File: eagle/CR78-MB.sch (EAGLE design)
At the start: 29 parts, among them IC1 40106N, Q1 2N3904, Q510 2N3904, Q518 2N3904, Q7 2N3904

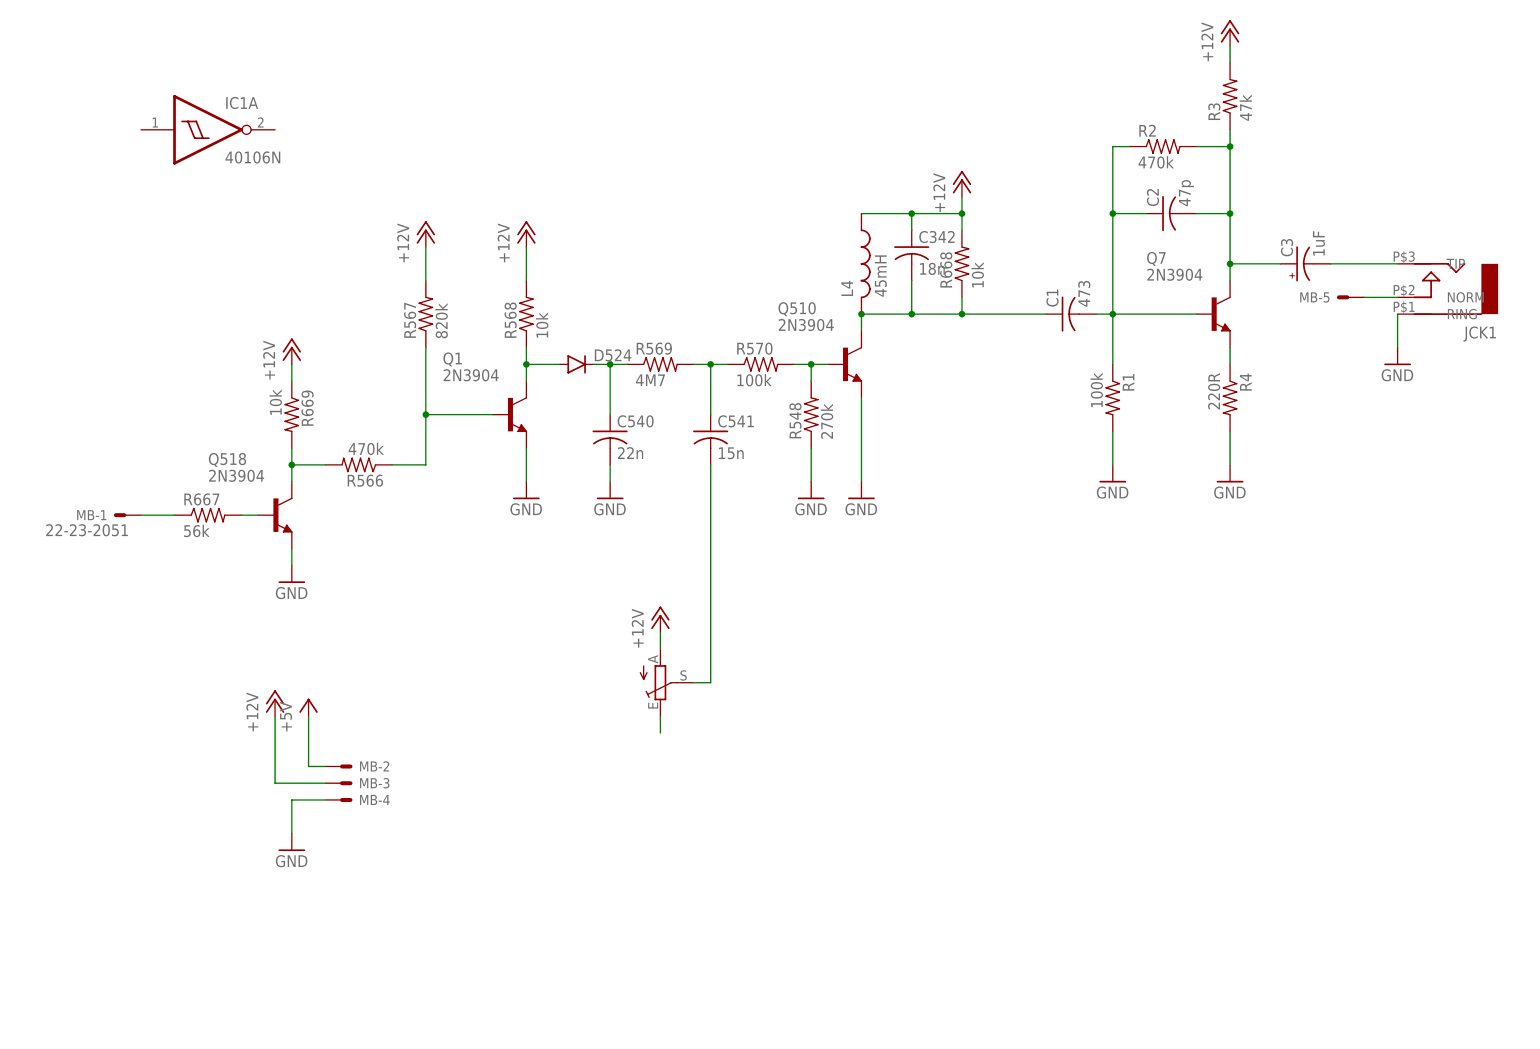
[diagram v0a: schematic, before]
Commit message: schemo
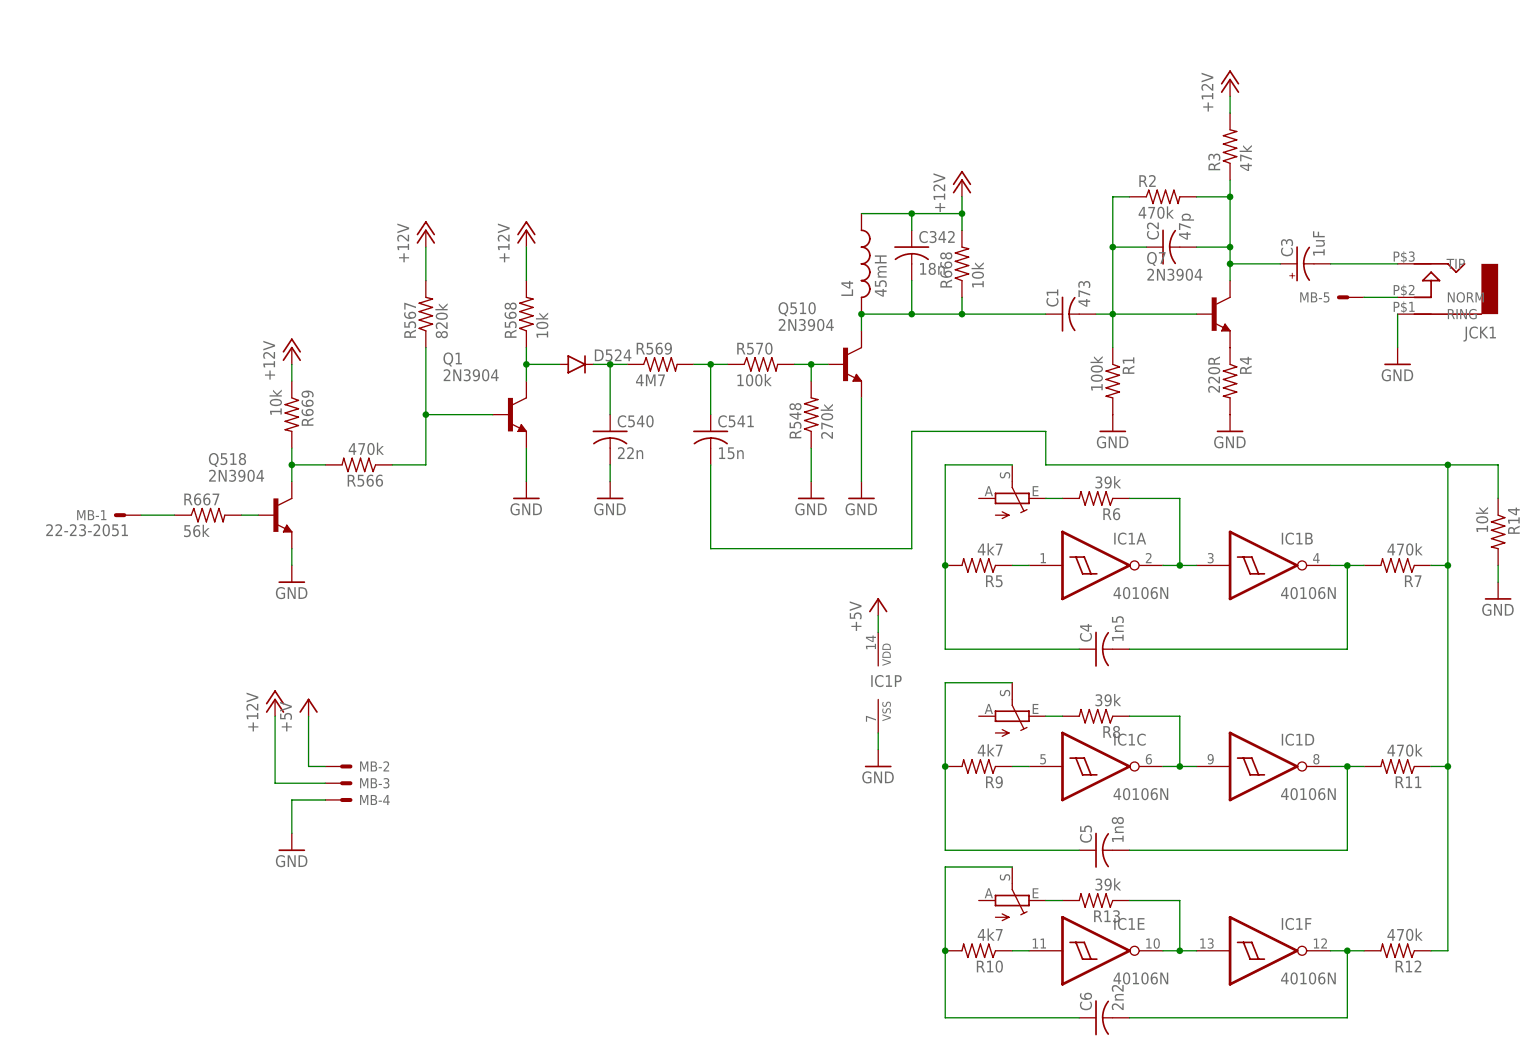
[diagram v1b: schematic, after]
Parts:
- removed VR63: 50KB, TR808clone:TRIM_EU-B64Y
- added C4: 1n5, rcl:C-US050-025X075
- added C5: 1n8, rcl:C-US050-025X075
- added C6: 2n2, rcl:C-US050-025X075
- added R10, R5, R9: 4k7, rcl:R-US_0207/7
- added R11, R12, R7: 470k, rcl:R-US_0207/7
- added R13, R6, R8: 39k, rcl:R-US_0207/7
- added R14: 10k, rcl:R-US_0207/7
- added VR1, VR2, VR3: 20K, TR808clone:TRIM_EU-B64Y
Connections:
- new net N$10: IC1E.O, IC1F.I, R13.1
- new net N$11: C5.2, IC1D.O, R11.2
- new net N$14: C6.2, IC1F.O, R12.2
- new net N$22: C4.2, IC1B.O, R7.2
- new net N$23: R6.2, VR1.E
- new net N$25: R8.2, VR2.E
- new net N$26: R13.2, VR3.E
- new net N$28: C4.1, R5.2, VR1.S
- new net N$29: C5.1, R9.2, VR2.S
- new net N$30: C6.1, R10.2, VR3.S
- new net N$5: IC1A.O, IC1B.I, R6.1
- new net N$6: IC1C.O, IC1D.I, R8.1
- new net N$8: IC1C.I, R9.1
- new net N$9: IC1E.I, R10.1
- net +12V: no longer VR63.A
- net +5V: now also IC1P.VDD
- net GND: now also IC1P.VSS, R14.2
- net N$17: now also IC1A.I, R5.1; no longer C541.2, VR63.S
- net N$3: now also C541.2, R11.1, R12.1, R14.1, R7.1; no longer VR63.E
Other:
- moved on the sheet: C2, IC1A, R1, R2, R3, R4
